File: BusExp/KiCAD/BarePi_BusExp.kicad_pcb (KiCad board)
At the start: 2 copper layers, 52 x 36 mm, 4 parts, among them J1 IN, J2 OUT, J3 IN, J4 OUT

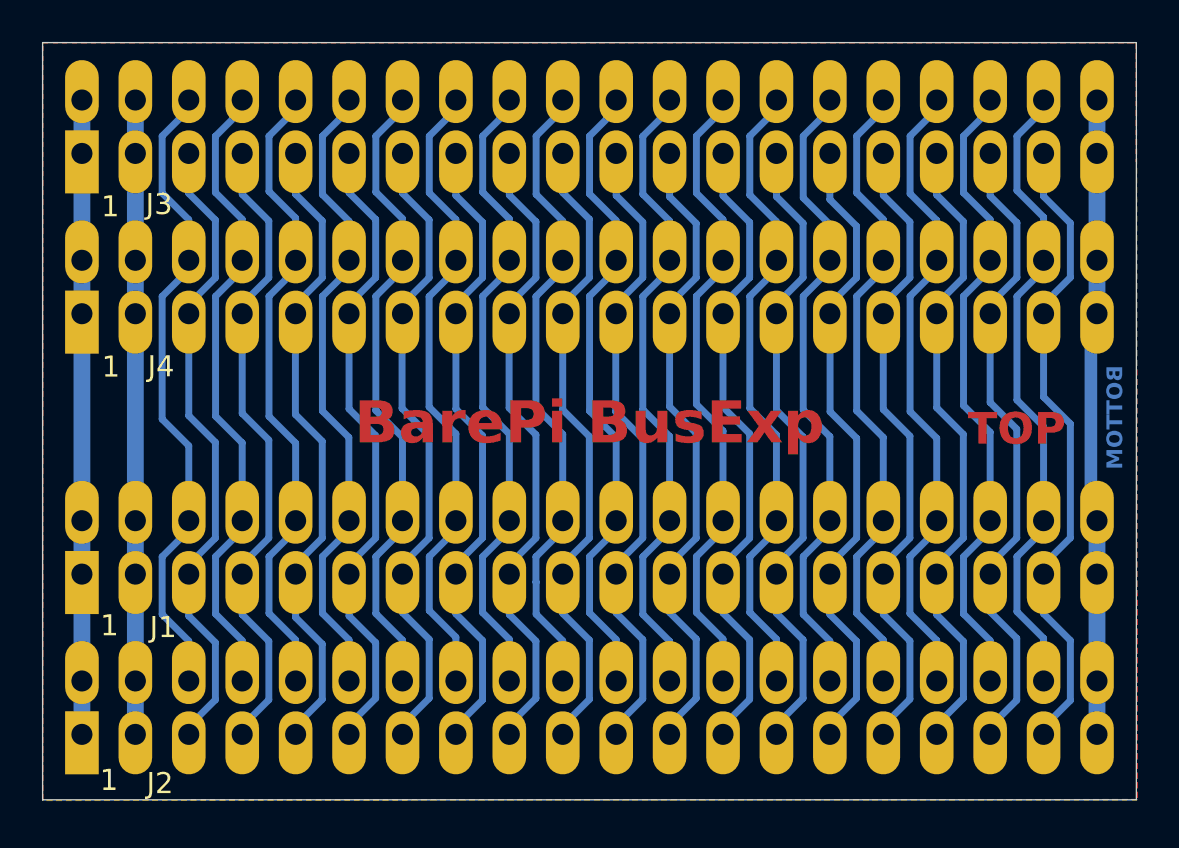
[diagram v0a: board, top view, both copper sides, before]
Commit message: init
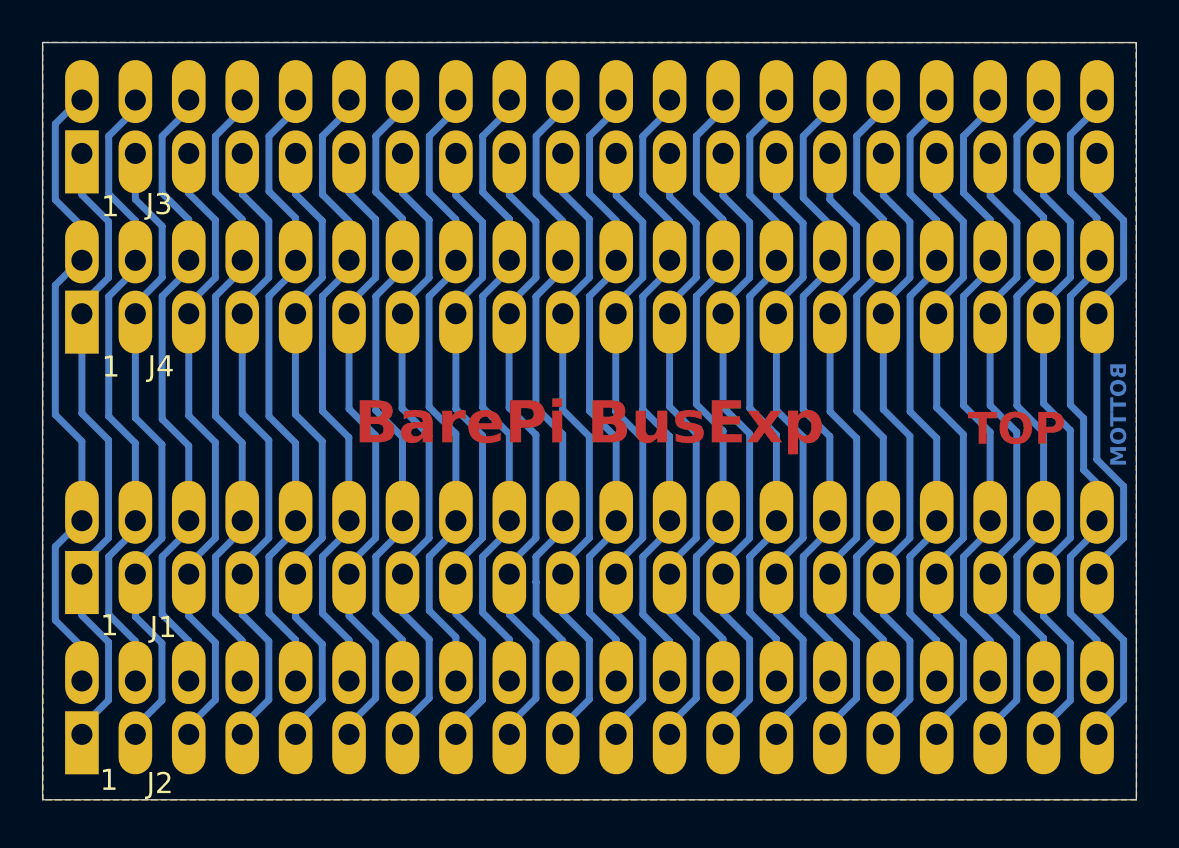
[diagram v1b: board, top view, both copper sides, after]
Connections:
- J1 pad 1: /5V -> /5V_1
- J1 pad 2: /5V -> /5V_2
- J1 pad 3: /3V3 -> /3V3_1
- J1 pad 39: /GND -> /GND_1
- J1 pad 4: /3V3 -> /3V3_2
- J1 pad 40: /GND -> /GND_2
- J2 pad 1: /5V -> /5V_1
- J2 pad 2: /5V -> /5V_2
- J2 pad 3: /3V3 -> /3V3_1
- J2 pad 39: /GND -> /GND_1
- J2 pad 4: /3V3 -> /3V3_2
- J2 pad 40: /GND -> /GND_2
- J3 pad 1: /5V -> /5V_1
- J3 pad 2: /5V -> /5V_2
- J3 pad 3: /3V3 -> /3V3_1
- J3 pad 39: /GND -> /GND_1
- J3 pad 4: /3V3 -> /3V3_2
- J3 pad 40: /GND -> /GND_2
- J4 pad 1: /5V -> /5V_1
- J4 pad 2: /5V -> /5V_2
- J4 pad 3: /3V3 -> /3V3_1
- J4 pad 39: /GND -> /GND_1
- J4 pad 4: /3V3 -> /3V3_2
- J4 pad 40: /GND -> /GND_2
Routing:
- net /GND_1: track 0.00 -> 31.2 mm
- net /GND_2: track 0.00 -> 31.2 mm
- net /5V_2: track 0.00 -> 30.9 mm
- net /3V3_1: track 0.00 -> 30.8 mm
- net /5V_1: track 0.00 -> 30.8 mm
- net /3V3_2: track 0.00 -> 30.8 mm
- net /GND: track 30.4 -> 0.00 mm
- net /5V: track 30.2 -> 0.00 mm
- net /3V3: track 30.2 -> 0.00 mm
- added copper zone on B.Cu, net /GND_1
- added copper zone on F.Cu, net /GND_1
- removed copper zone on B.Cu, net /GND
- removed copper zone on F.Cu, net /GND
